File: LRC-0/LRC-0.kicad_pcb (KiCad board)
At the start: 4 copper layers, 60 x 40 mm, 58 parts, among them J1 USB_C_Receptacle_USB2.0_14P, J2 Battery, J3 Conn_01x10, J4 SMA, J5 u.FL, SW1 EN, SW2 BOOT, SW3 SW_SPDT, U1 AP7361C-33E, U2 TVS1400DRV, U3 BQ24075RGT, U4 ESP32-C6-MINI-1, U5 SX1262IMLTRT, U6 4259-63, U8 4259-63, Y1 TX32-33015S-32.000-X-R

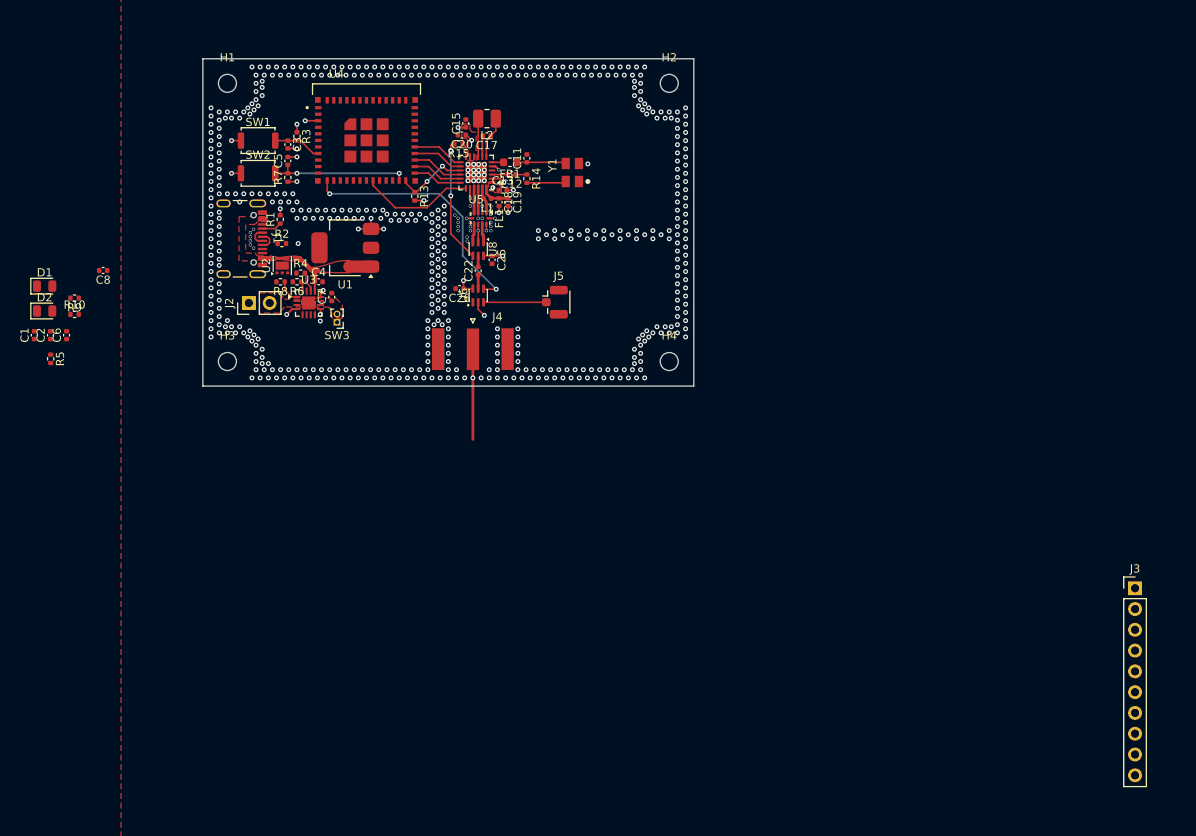
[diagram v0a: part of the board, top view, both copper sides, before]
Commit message: stitching
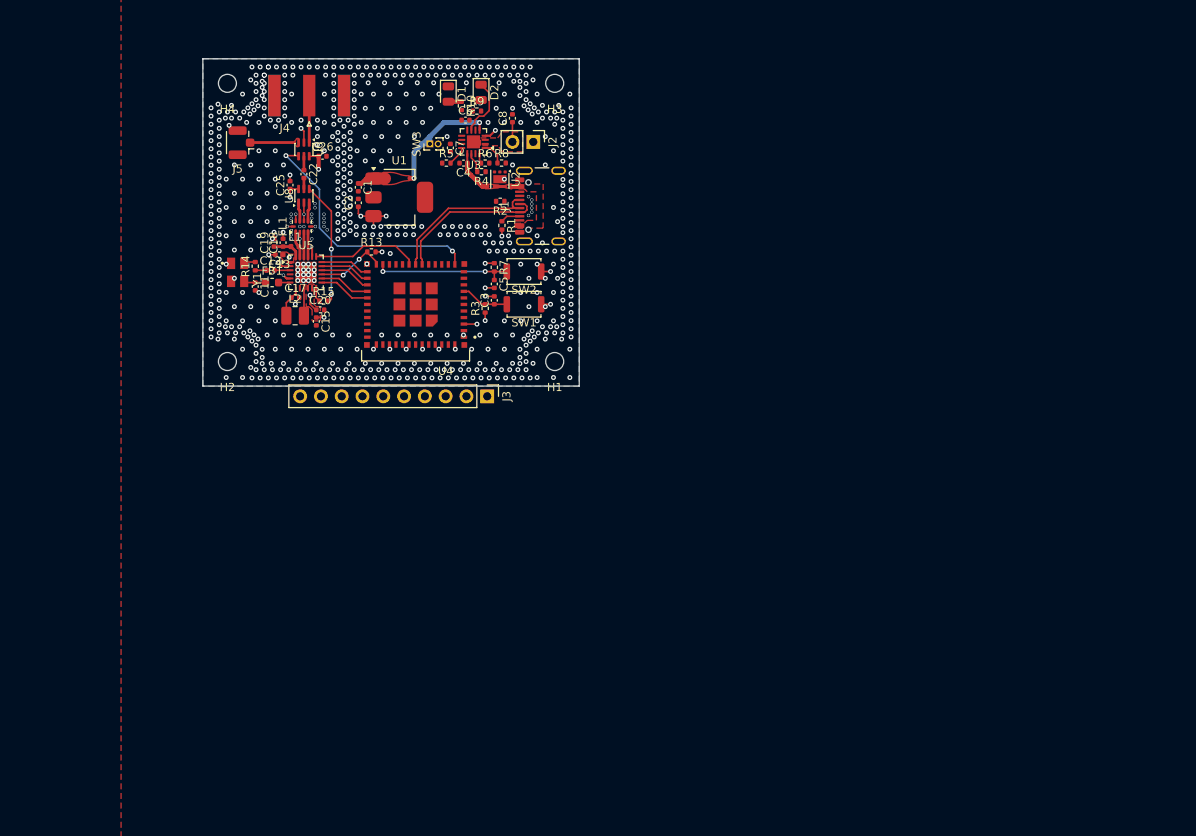
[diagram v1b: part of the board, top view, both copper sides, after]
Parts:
- moved J3 82.6 mm to (34.8, 41.2), turned to -90 degrees
- moved H2 63.8 mm to (3.00, 37.0), turned to 180 degrees
- moved H4 63.8 mm to (3.00, 3.00), turned to 180 degrees
- moved D2 59.7 mm to (34.0, 4.10), turned to -90 degrees
- moved C6 55.4 mm to (32.1, 7.50), turned to 0 degrees
- moved D1 54.6 mm to (30.0, 4.31), turned to -90 degrees
- moved R9 54.2 mm to (33.5, 6.39), turned to 0 degrees
- moved R5 54.0 mm to (29.8, 12.8), turned to 0 degrees
- moved R10 53.7 mm to (31.6, 5.76), turned to -90 degrees
- moved C8 53.4 mm to (37.8, 7.27), turned to 90 degrees
- moved H1 52.5 mm to (43.0, 37.0), turned to 180 degrees
- moved H3 52.5 mm to (43.0, 3.00), turned to 180 degrees
- moved J5 43.8 mm to (4.25, 10.2), turned to 180 degrees
- moved C1 43.5 mm to (19.0, 15.7), turned to -90 degrees
- moved Y1 42.7 mm to (4.25, 26.1), turned to -90 degrees
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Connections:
- net GND renamed Earth_Protective
- C1 pad 1: VBUS -> VCC
- U1 pad 1: VBUS -> VCC
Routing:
- net VCC: track 0.00 -> 19.6 mm, vias 0 -> 2
- net /D+: track 2.44 -> 19.7 mm
- net /D-: track 2.44 -> 18.9 mm
- net Net-(D2-K): track 0.00 -> 7.20 mm
- net /ANT2: track 10.6 -> 5.73 mm
- net VBUS: track 11.1 -> 7.62 mm
- net Net-(Y1-OUTPUT): track 5.02 -> 1.62 mm
- net Net-(Y1-VDC): track 6.09 -> 2.69 mm
- net /BAT+: track 0.00 -> 2.41 mm
- net /ANT1: track 7.68 -> 5.48 mm
- net +3V3: track 15.6 -> 17.8 mm
- net Earth_Protective: track 22.6 -> 20.7 mm, vias 571 -> 678
- net Net-(D1-A): track 0.00 -> 1.60 mm
- net Net-(U3-ILIM): track 0.93 -> 2.41 mm, vias 1 -> 0
- net Net-(U5-VREG): track 5.12 -> 3.84 mm
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- added copper zone on F.Cu, net /ANT1
- added copper zone on B.Cu, net Earth_Protective
- added copper zone on F.Cu, net VCC
- removed copper zone on F.Cu, net VOUT
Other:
- board size 60 x 40 mm -> 46 x 40 mm

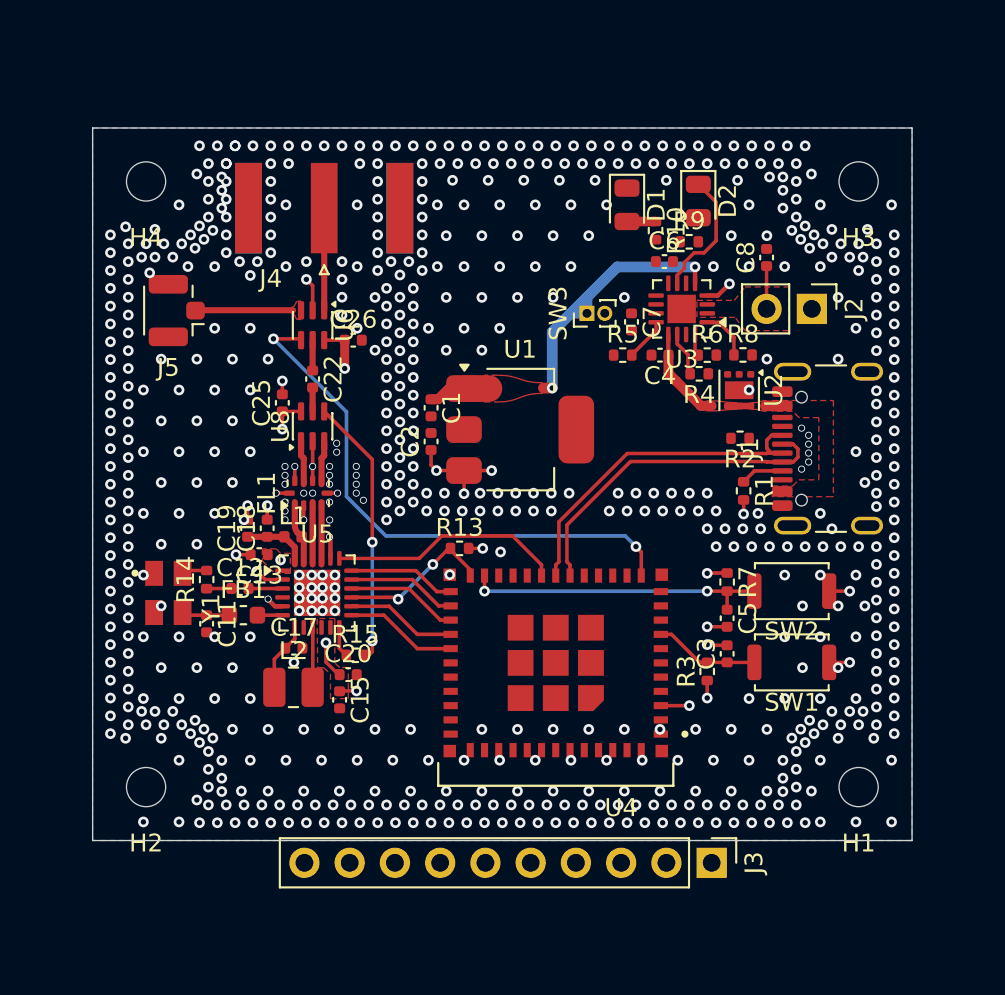
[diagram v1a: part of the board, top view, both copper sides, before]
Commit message: bom and jlcpcb quote
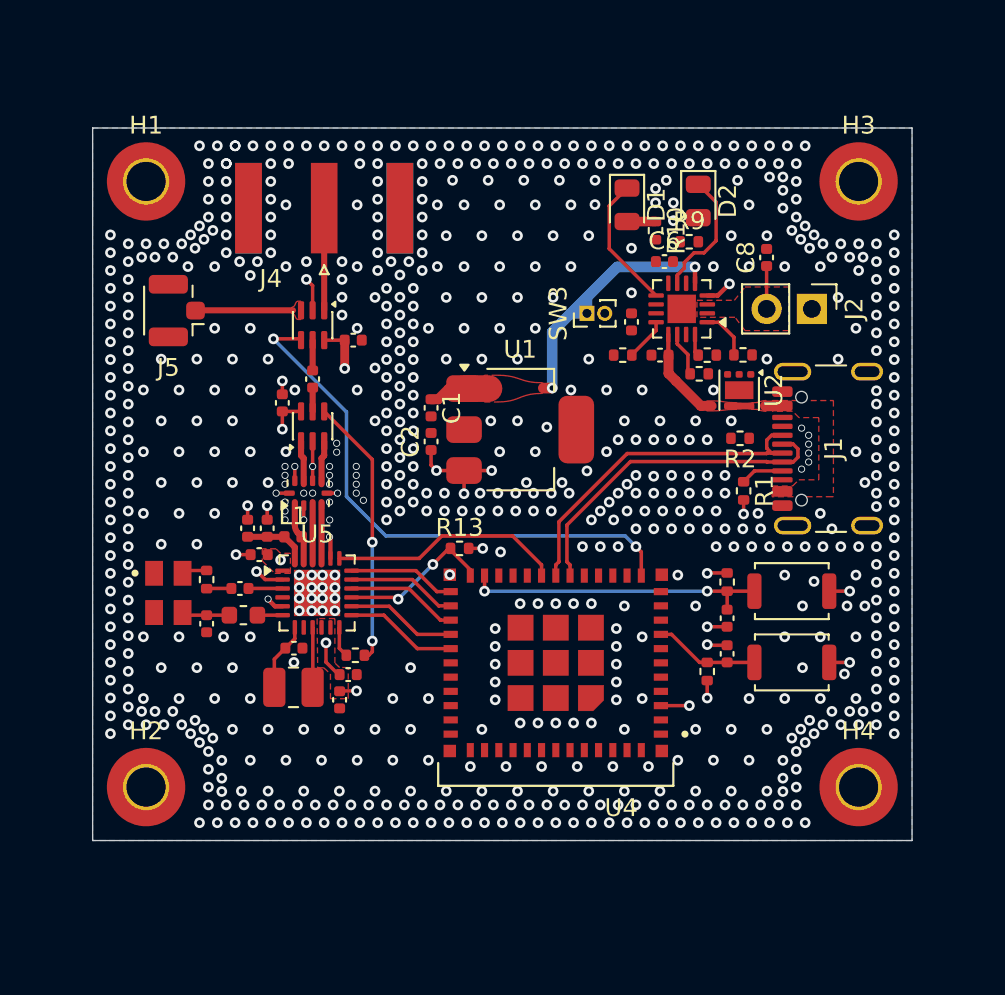
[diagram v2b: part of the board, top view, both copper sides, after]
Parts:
- removed J3: Conn_01x10, Connector_PinHeader_2.54mm:PinHeader_1x10_P2.54mm_Vertical
- H1, H2, H3, H4: value MountingHole -> MountingHole_Pad_MP; footprint MountingHole:MountingHole_2.2mm_M2 -> MountingHole:MountingHole_2.2mm_M2_Pad_TopOnly
- moved H1 52.5 mm to (3.00, 3.00), turned to 0 degrees
- moved H4 52.5 mm to (43.0, 37.0), turned to 0 degrees
- turned H2 to 0 degrees
- turned H3 to 0 degrees
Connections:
- C11 pad 2: Earth_Protective -> unconnected-(C11-Pad2)
- Y1 pad 1: Earth_Protective -> Net-(Y1-GND)
- Y1 pad 2: Earth_Protective -> Net-(Y1-GND)
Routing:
- net Net-(D1-K): track 0.00 -> 7.53 mm
- net Earth_Protective: vias 678 -> 725
